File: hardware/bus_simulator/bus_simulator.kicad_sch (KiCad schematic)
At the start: 68 parts, among them J1 I2C_LCD, J2 Encoder, Q1 BUK7880-55A, Q2 BUK7880-55A, SW1 SW_Push, SW10 SW_Push, SW11 SW_Push, SW12 SW_Push, SW2 SW_Push, SW3 SW_Push, SW4 SW_Push, SW5 SW_Push, SW6 SW_Push, SW7 SW_Push, SW8 SW_Push, SW9 SW_Push, U1 RaspberryPi_Pico, U2 74HC595, U3 74HC595, U4 74HC595

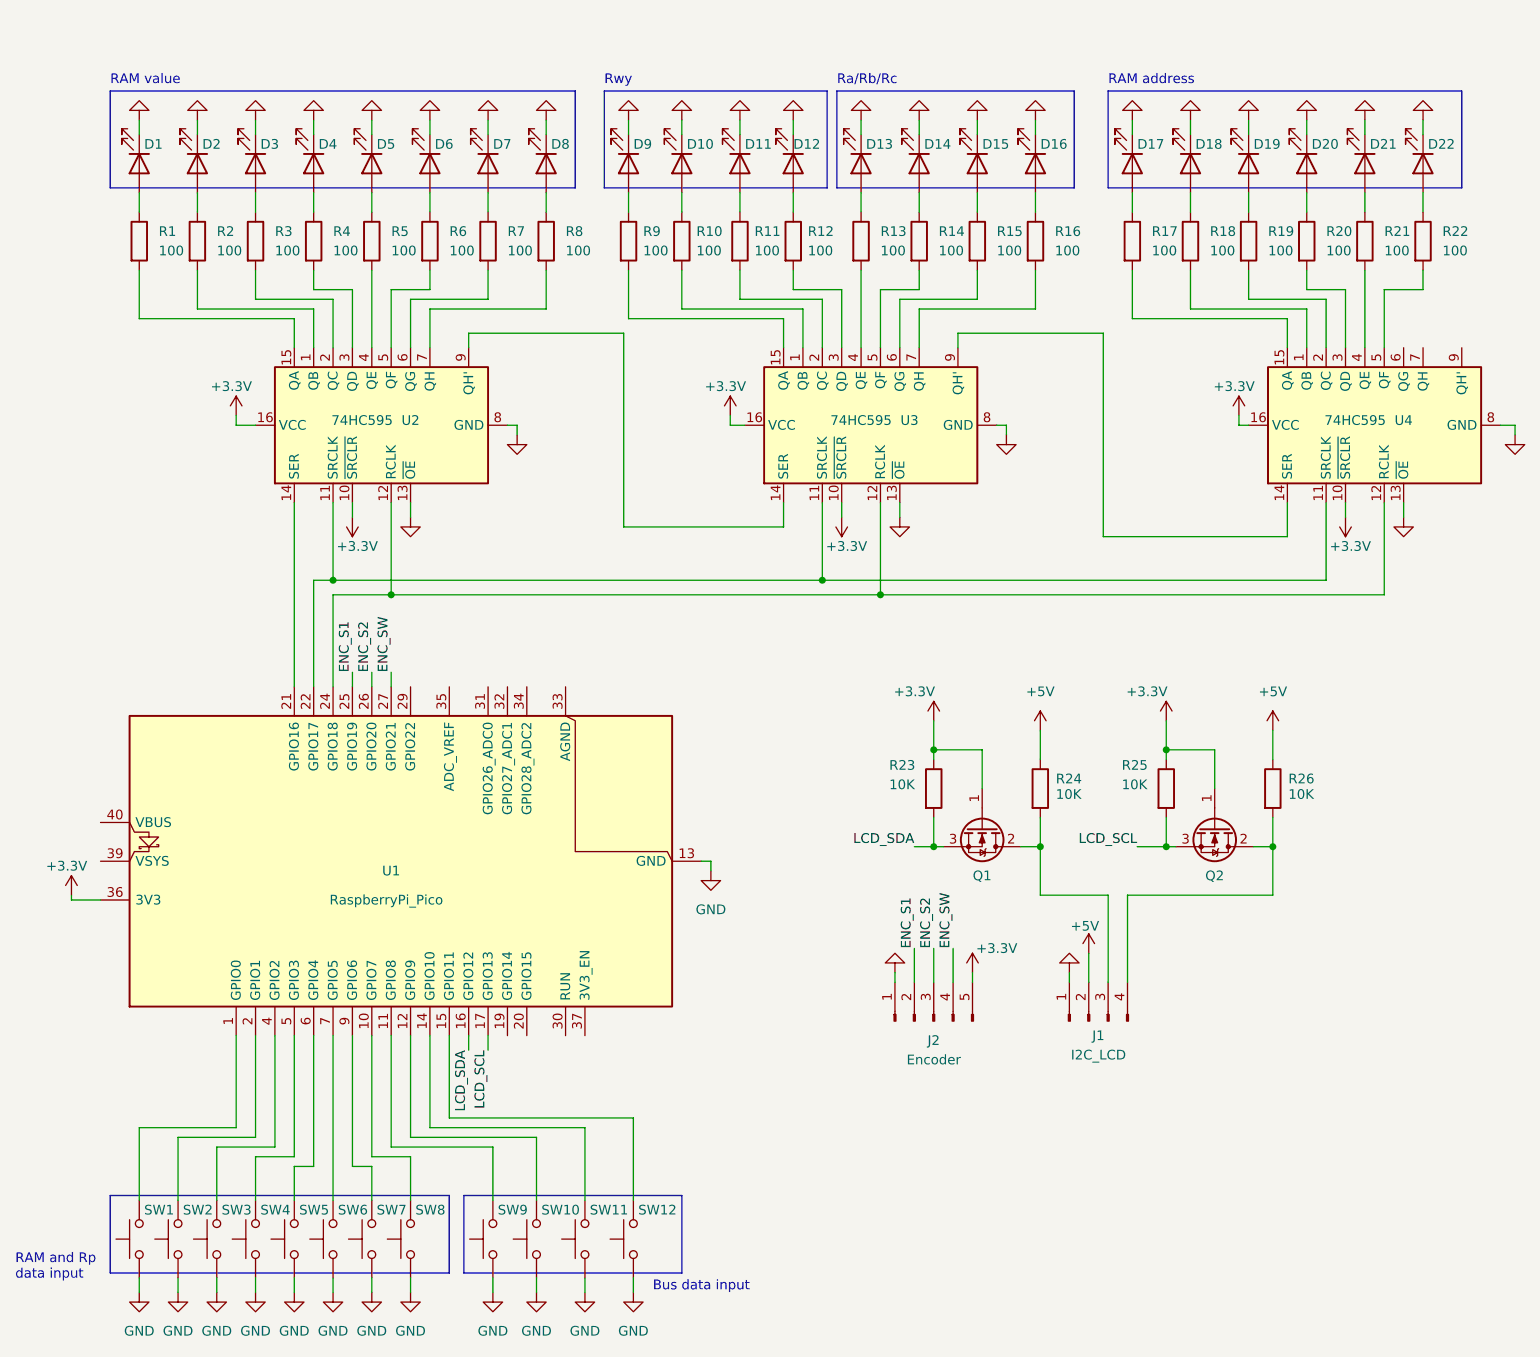
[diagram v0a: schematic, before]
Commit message: Fixed typos and removed old comments
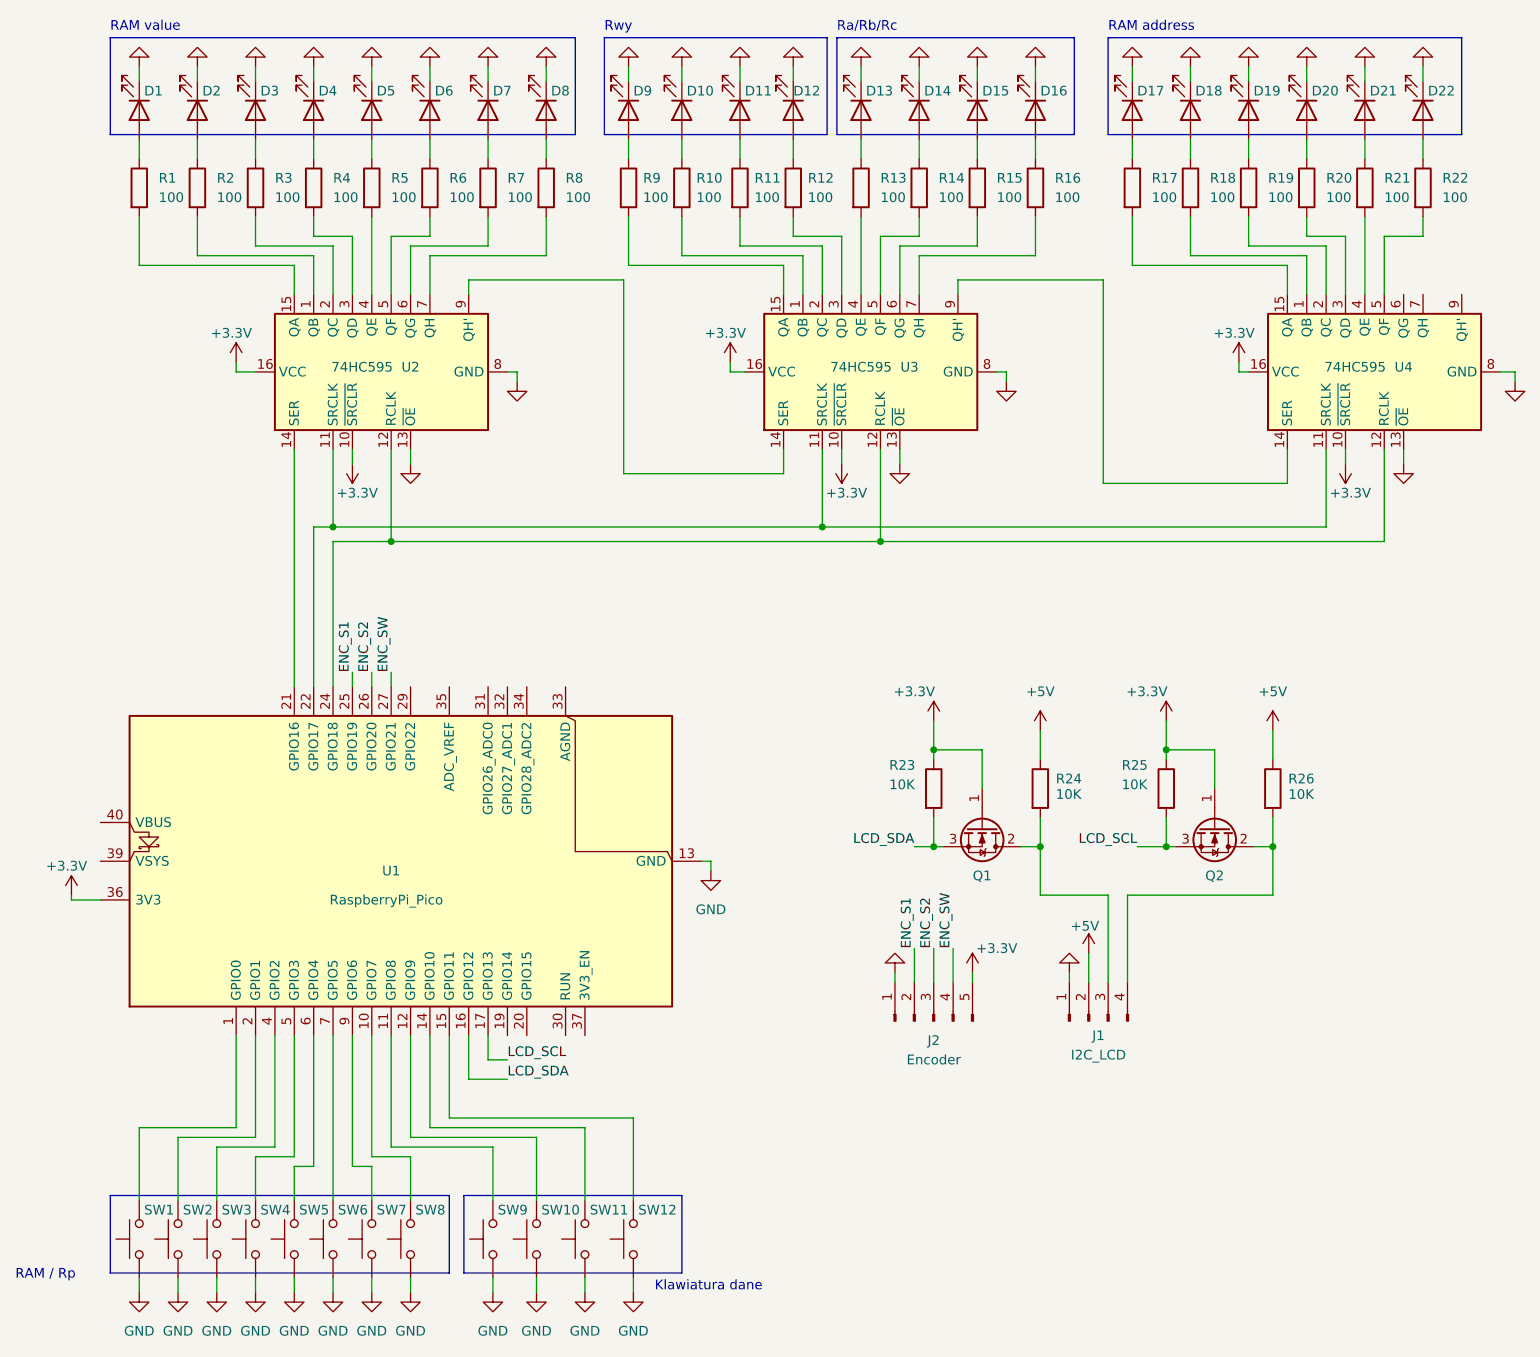
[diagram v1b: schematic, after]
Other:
- note added: "Klawiatura dane"
- note added: "RAM / Rp"
- note removed: "Bus data input"
- note removed: "RAM and Rp data input"
- moved on the sheet: D1, D10, D11, D12, D13, D14, D15, D16, D17, D18, D19, D2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

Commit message: Schematic fixes
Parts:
- J1: footprint (none) -> Connector_JST:JST_XH_B4B-XH-A_1x04_P2.50mm_Vertical
- J2: footprint (none) -> Connector_JST:JST_XH_B5B-XH-A_1x05_P2.50mm_Vertical
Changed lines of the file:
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@@
 	(label "LCD_SDA"
 		(at 168.91 125.73 180)
-		(fields_autoplaced yes)
 		(effects
 			(font
@@
 	(label "ENC_S1"
 		(at 95.25 102.87 90)
-		(fields_autoplaced yes)
 		(effects
 			(font
@@
 	(label "ENC_S2"
 		(at 97.79 102.87 90)
-		(fields_autoplaced yes)
 		(effects
 			(font
@@
 	(label "ENC_SW"
 		(at 173.99 139.065 90)
-		(fields_autoplaced yes)
 		(effects
 			(font
@@
 	(label "LCD_SCL"
 		(at 198.12 125.73 180)
-		(fields_autoplaced yes)
 		(effects
 			(font
@@
 	(label "ENC_S1"
 		(at 168.91 139.065 90)
-		(fields_autoplaced yes)
 		(effects
 			(font
@@
 	(label "LCD_SDA"
 		(at 115.57 156.21 0)
-		(fields_autoplaced yes)
 		(effects
 			(font
@@
 	(label "LCD_SCL"
 		(at 115.57 153.67 0)
-		(fields_autoplaced yes)
 		(effects
 			(font
@@
 	(label "ENC_S2"
 		(at 171.45 139.065 90)
-		(fields_autoplaced yes)
 		(effects
 			(font
@@
 	(label "ENC_SW"
 		(at 100.33 102.87 90)
-		(fields_autoplaced yes)
 		(effects
 			(font
@@
 			)
 		)
-		(property "Footprint" ""
+		(property "Footprint" "Connector_JST:JST_XH_B4B-XH-A_1x04_P2.50mm_Vertical"
 			(at 191.77 148.59 0)
 			(effects
@@
 			)
 		)
-		(property "Footprint" ""
+		(property "Footprint" "Connector_JST:JST_XH_B5B-XH-A_1x05_P2.50mm_Vertical"
 			(at 171.45 148.59 0)
 			(effects
